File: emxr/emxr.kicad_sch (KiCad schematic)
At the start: 10 parts, among them J101 POWER, J102 DSP_PW, J103 Bus Conn, J104 GEQ_L_PRE, J105 GEQ_L_POST, J106 GEQ_R_PRE, J107 GEQ_R_POST, J108 AUDIO_OUT

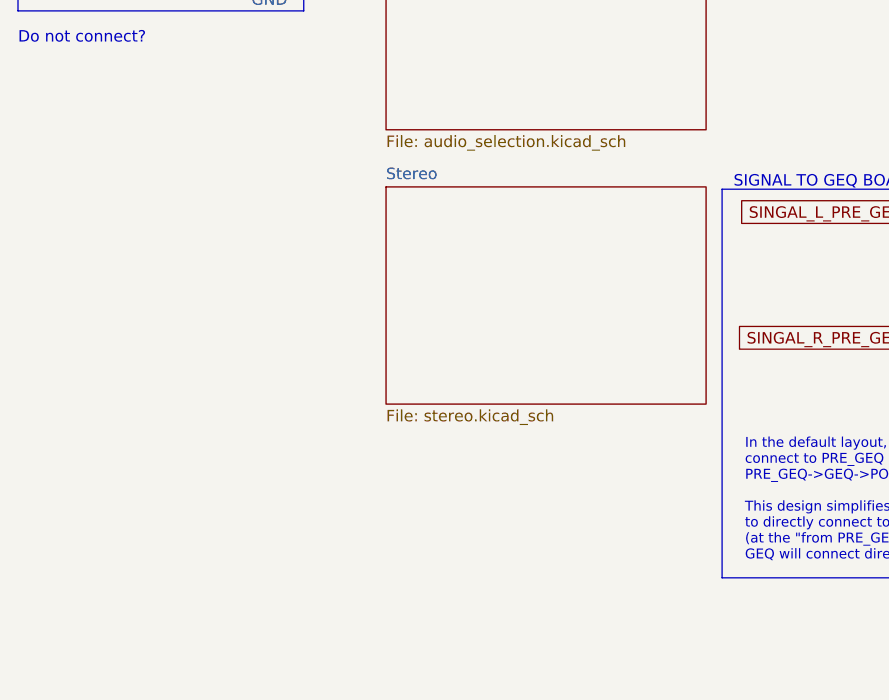
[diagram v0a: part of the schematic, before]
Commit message: replicated layout
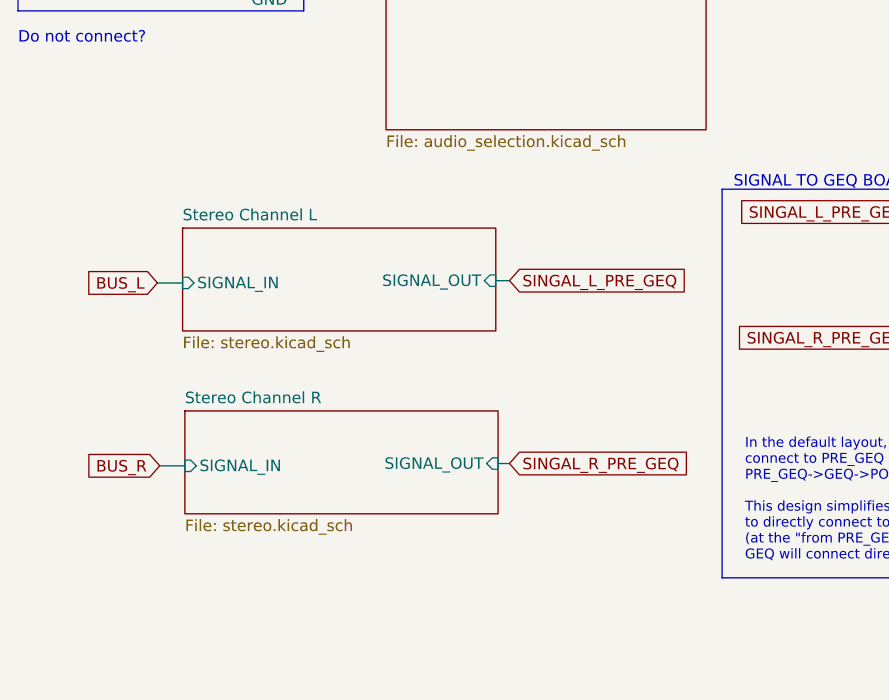
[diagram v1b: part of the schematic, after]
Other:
- sheet Stereo renamed Stereo Channel L
- added sheet Stereo Channel R (stereo.kicad_sch)
- sheet Stereo Channel L ports: added SIGNAL_IN, SIGNAL_OUT; removed none

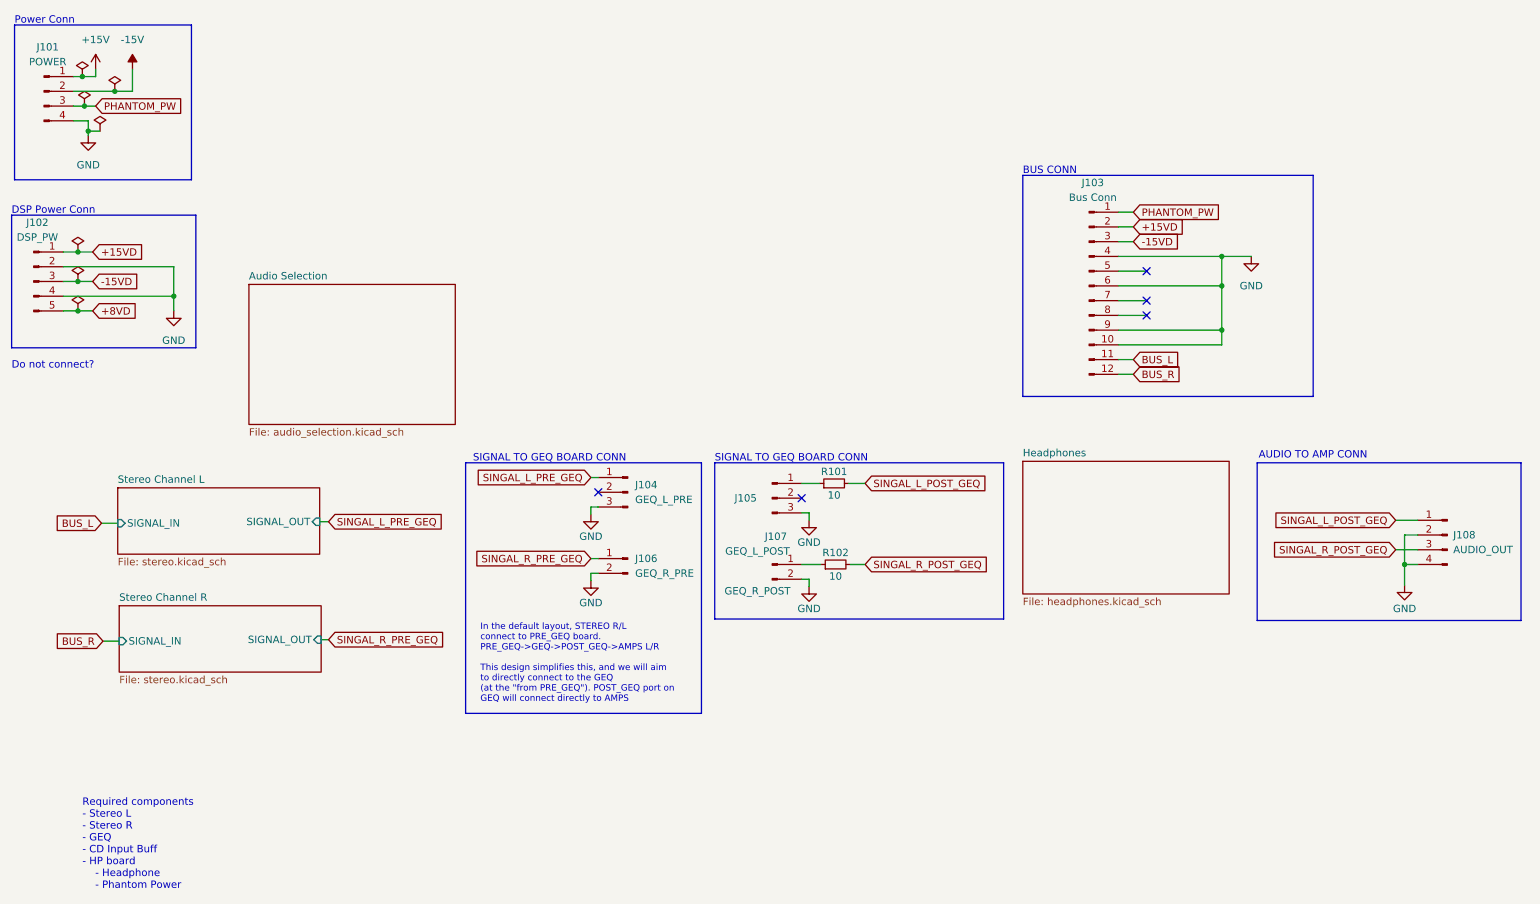
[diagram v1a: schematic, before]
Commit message: more routing and reshuffling
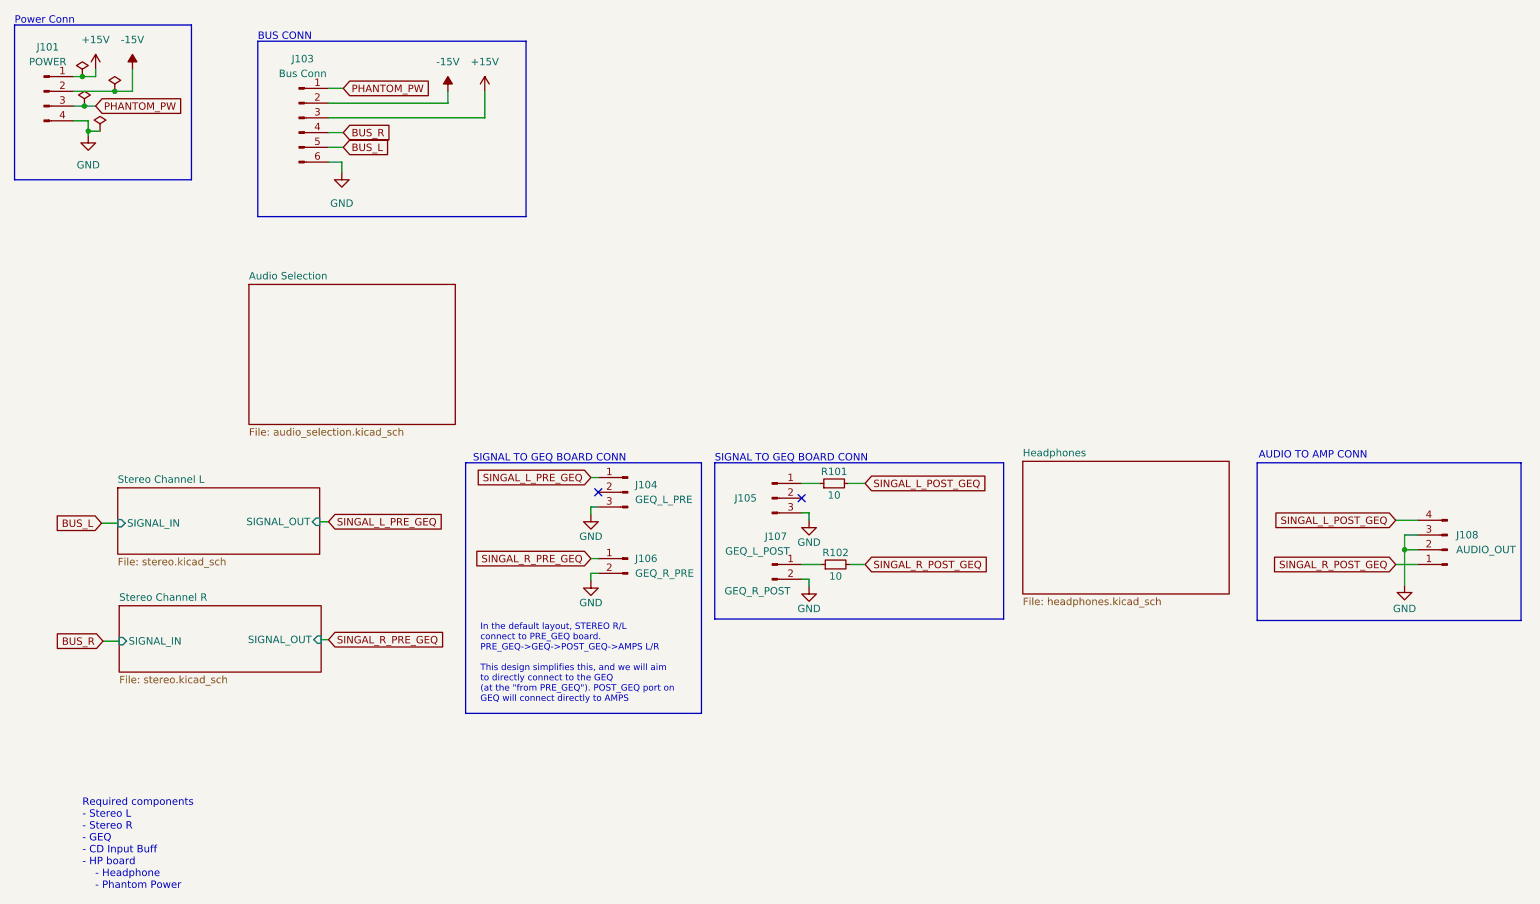
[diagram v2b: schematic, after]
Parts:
- removed J102: DSP_PW, Connector_JST:JST_XH_B5B-XH-A_1x05_P2.50mm_Vertical, symbol Connector:Conn_01x05_Male
- removed J103: Bus Conn, Connector_PinHeader_2.54mm:PinHeader_1x12_P2.54mm_Vertical, symbol Connector:Conn_01x12_Male
- added J103: Bus Conn, Connector_JST:JST_XH_B6B-XH-A_1x06_P2.50mm_Vertical, symbol Connector:Conn_01x06_Male
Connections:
- net +15V: now also J103.3 (Pin_3)
- net -15V: now also J103.2 (Pin_2)
- net BUS_L: now also J103.5 (Pin_5)
- net BUS_R: now also J103.4 (Pin_4)
- net GND: now also J108.3 (Pin_3), J103.6 (Pin_6); no longer J108.4 (Pin_4)
- net PHANTOM_PW: now also J103.1 (Pin_1)
- net SINGAL_L_POST_GEQ: now also J108.4 (Pin_4); no longer J108.1 (Pin_1)
- net SINGAL_R_POST_GEQ: now also J108.1 (Pin_1); no longer J108.3 (Pin_3)
- no-connect marks 5 -> 2
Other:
- note removed: "DSP Power Conn"
- note removed: "Do not connect?"
- moved on the sheet: J108
